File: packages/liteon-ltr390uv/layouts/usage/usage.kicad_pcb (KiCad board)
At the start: 2 copper layers, 5 parts

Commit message: Clean PR: Only include packages from package-todos.md
- Updated layouts and parts for packages listed in package-todos.md only
- Includes adi-ad5693r, adi-adbms6822, adi-adbms6830, adi-adxl375, adi-ltc4316
- Updated ams-tsl2591, aosong-aht20, bosch sensors, diodes-inc, espressif
- Updated infineon, invensense, issi, liteon, macroblock, maxim components
- Updated memsic, microchip, rohm, nxp, opsco, st, ti, usb-connectors
- Renamed pjrc-teensy_4_1 to pjrc-teensy-4-1 (hyphen naming convention)
- Updated realtek-rtl8305nb

Removed 64+ packages that were not listed in package-todos.md to keep
PR focused only on packages that are being tracked for review.
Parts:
- R2, R3: value 10kΩ ±1% 62.5mW -> 4.7kΩ ±1% 62.5mW; footprint UNI_ROYAL_0402WGF1002TCE:R0402 -> UNI_ROYAL_0402WGF4701TCE:R0402
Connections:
- net gnd renamed GND
- net hv renamed VCC

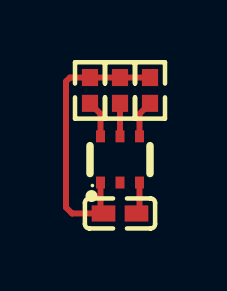
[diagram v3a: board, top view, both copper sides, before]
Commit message: scrub layouts
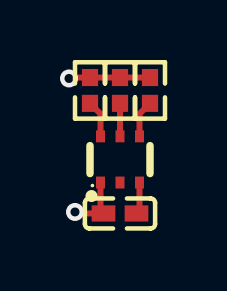
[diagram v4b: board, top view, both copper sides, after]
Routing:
- net VCC: track 9.46 -> 4.75 mm, vias 0 -> 2
